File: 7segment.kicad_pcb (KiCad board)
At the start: 2 copper layers, 31.8 x 23.4 mm, 12 parts, among them J1 VCC, J2 IN_UP, J3 GND, J4 IN_DOWN, U1 LTD-2601G, U2 ATmega328P-AU

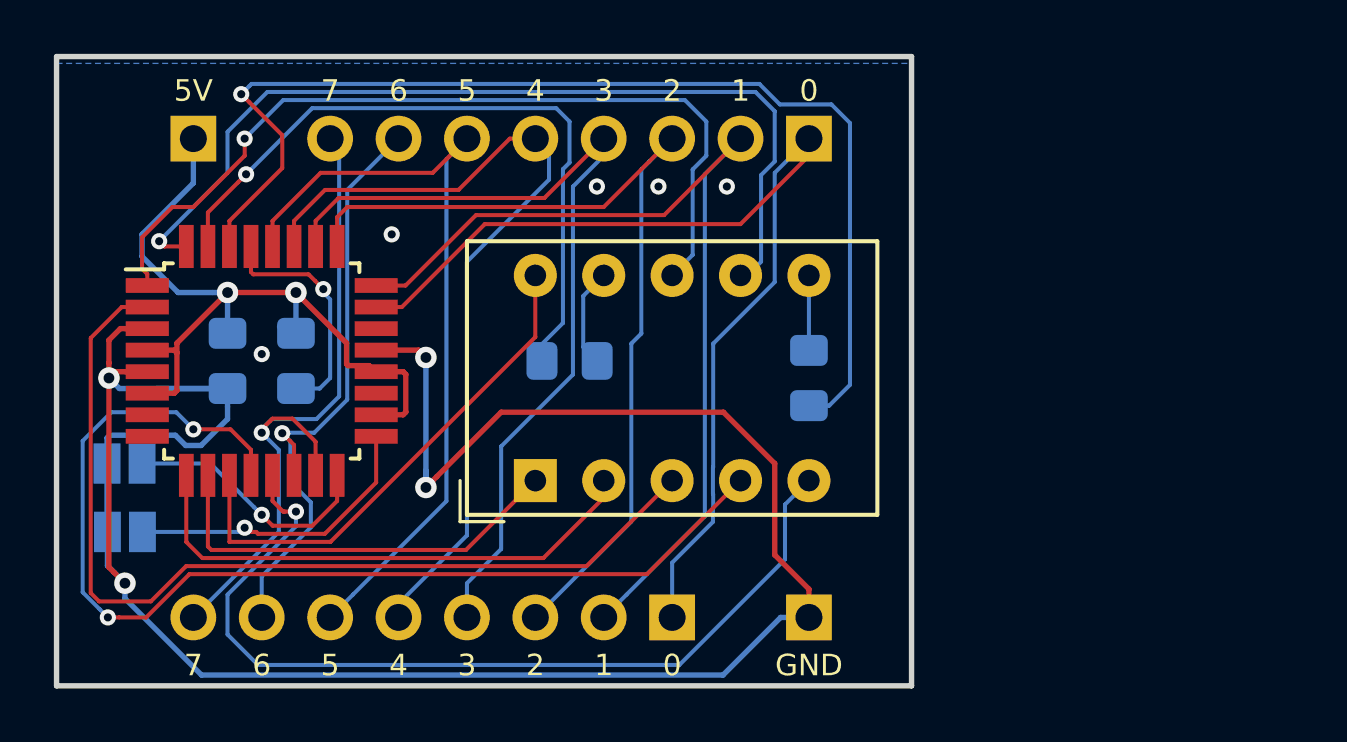
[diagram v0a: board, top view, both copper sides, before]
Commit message: Revision B
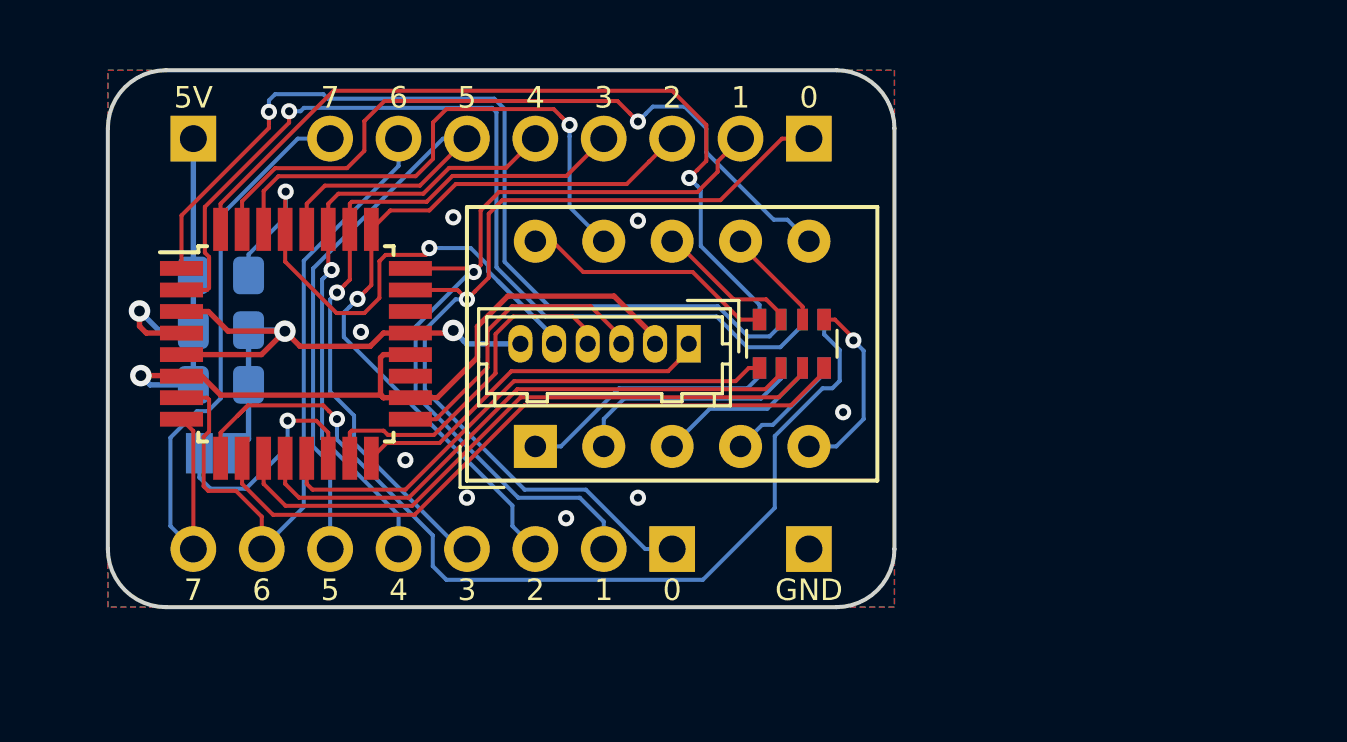
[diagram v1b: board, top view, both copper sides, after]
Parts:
- removed JP1: DIM, Jumper:SolderJumper-2_P1.3mm_Open_Pad1.0x1.5mm
- removed R1, R2: 220, Resistor_SMD:R_0805_2012Metric_Pad1.15x1.40mm_HandSolder
- added C2: 0.1uF, Capacitor_SMD:C_0805_2012Metric_Pad1.15x1.40mm_HandSolder, B.Cu at (64.5, 47.2)
- added J5: AVR-ISP-6, Connector_Hirose:Hirose_DF13-06P-1.25DSA_1x06_P1.25mm_Vertical, F.Cu at (81.9, 45.7)
- added RN1: 220, Resistor_SMD:R_Array_Convex_4x0603, B.Cu at (85.7, 45.7)
- added RN2: 220, Resistor_SMD:R_Array_Convex_4x0603, F.Cu at (85.7, 45.7)
- moved JP2 4.49 mm to (64.4, 49.8), turned to 0 degrees
- moved R3 4.22 mm to (64.5, 43.2), turned to 0 degrees
- moved J3 2.54 mm to (86.4, 53.3), turned to 90 degrees
- moved J4 2.54 mm to (81.3, 53.3)
- moved U2 1.42 mm to (67.3, 45.7)
- moved U1 1.27 mm to (76.2, 49.5)
- moved C1 1.17 mm to (64.5, 45.2), turned to 0 degrees
- turned J1 to 90 degrees
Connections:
- net Net-(R3-Pad2) renamed ~RESET
- U1 pad 1: Net-(U1-Pad1) -> SEG_E
- U1 pad 10: Net-(U1-Pad10) -> SEG_F
- U1 pad 2: Net-(U1-Pad2) -> SEG_D
- U1 pad 3: Net-(U1-Pad3) -> SEG_C
- U1 pad 4: Net-(U1-Pad4) -> SEG_G
- U1 pad 5: Net-(U1-Pad5) -> SEG_DP
- U1 pad 6: Net-(R2-Pad2) -> D1
- U1 pad 7: Net-(U1-Pad7) -> SEG_A
- U1 pad 8: Net-(U1-Pad8) -> SEG_B
- U1 pad 9: Net-(R1-Pad2) -> D0
- U2 pad 1: Net-(U1-Pad8) -> Net-(RN1-Pad2)
- U2 pad 10: Net-(U1-Pad1) -> Net-(RN2-Pad8)
- U2 pad 11: Net-(U1-Pad10) -> Net-(RN2-Pad7)
- U2 pad 12: Net-(U1-Pad4) -> Net-(RN2-Pad6)
- U2 pad 13: Net-(U1-Pad5) -> Net-(RN2-Pad5)
- U2 pad 14: /IN6 -> Net-(JP2-Pad1)
- U2 pad 15: /IN7 -> MOSI
- U2 pad 16: Net-(JP1-Pad1) -> MISO
- U2 pad 17: Net-(JP2-Pad1) -> SCK
- U2 pad 2: Net-(U1-Pad3) -> Net-(RN1-Pad3)
- U2 pad 30: Net-(R2-Pad1) -> D0
- U2 pad 31: Net-(R1-Pad1) -> D1
- U2 pad 32: Net-(U1-Pad7) -> Net-(RN1-Pad1)
- U2 pad 7: Net-(U2-Pad7) -> /IN6
- U2 pad 8: Net-(U2-Pad8) -> /IN7
- U2 pad 9: Net-(U1-Pad2) -> Net-(RN1-Pad4)
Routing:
- net GND: track 89.7 -> 23.9 mm, vias 9 -> 10
- net Net-(R2-Pad1): track 42.0 -> 0.00 mm, vias 1 -> 0
- net Net-(U1-Pad4): track 40.8 -> 0.00 mm, vias 2 -> 0
- net Net-(RN1-Pad4): track 0.00 -> 35.8 mm, vias 0 -> 1
- net Net-(RN1-Pad3): track 0.00 -> 35.7 mm, vias 0 -> 1
- net Net-(U1-Pad3): track 35.6 -> 0.00 mm
- net Net-(U1-Pad7): track 34.2 -> 0.00 mm, vias 1 -> 0
- net Net-(RN1-Pad2): track 0.00 -> 34.1 mm, vias 0 -> 1
- net Net-(U1-Pad5): track 33.7 -> 0.00 mm, vias 1 -> 0
- net Net-(U1-Pad8): track 31.9 -> 0.00 mm, vias 1 -> 0
- net Net-(RN1-Pad1): track 0.00 -> 30.0 mm, vias 0 -> 1
- net D1: track 0.00 -> 27.4 mm, vias 0 -> 1
- net Net-(R1-Pad1): track 25.8 -> 0.00 mm, vias 1 -> 0
- net Net-(RN2-Pad8): track 0.00 -> 25.4 mm
- net Net-(RN2-Pad7): track 0.00 -> 23.5 mm
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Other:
- board size 31.8 x 23.4 mm -> 29.2 x 19.9 mm
- rule pad_to_mask_clearance: 0.12 -> 0.1
- board text added: "MISO"
- board text added: "MOSI"
- board text added: "RevB 2019 dev@hotkeysoft.net"
- board text added: "SCK"
- board text added: "VCC"
- board text added: "~RST"
- board text removed: "8 bit HEX Display RevA 2009 Dominic Thibodeau dev@hotkeysoft.net"
- board text removed: "DIM"

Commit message: Rev C
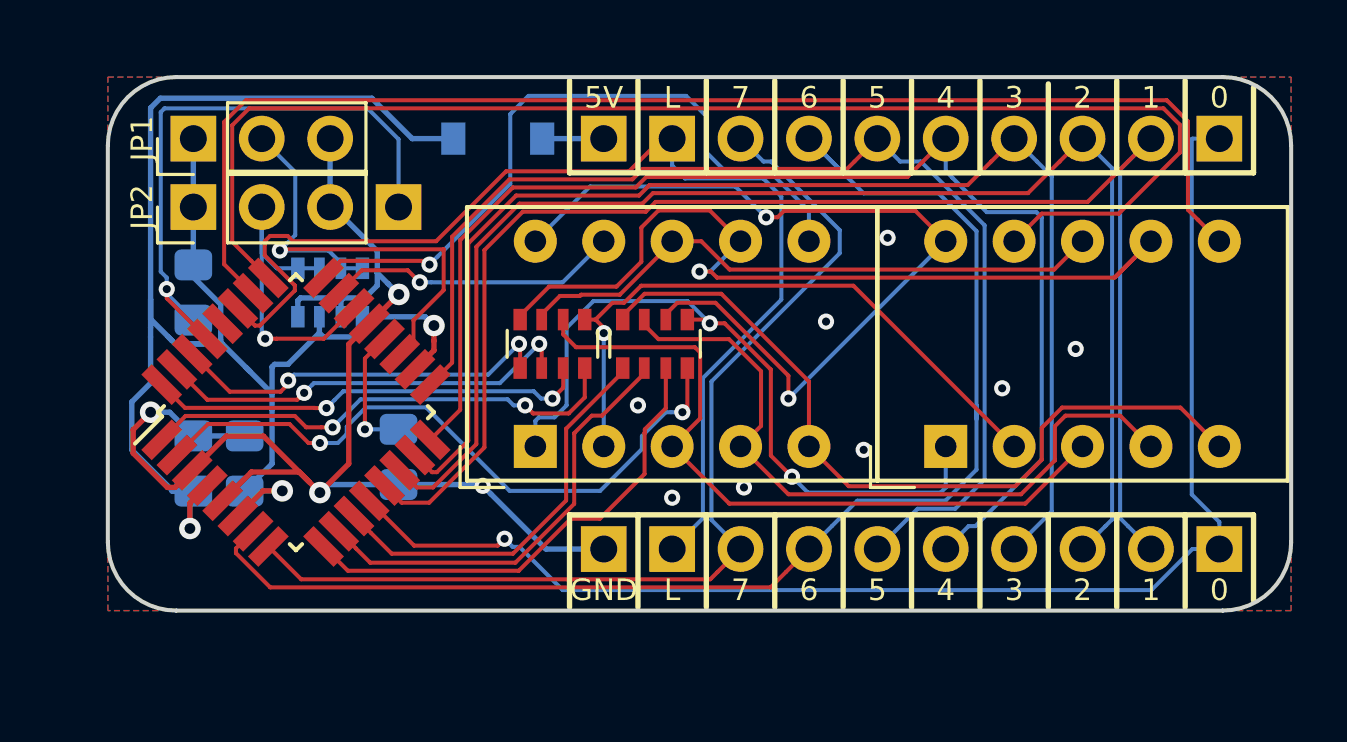
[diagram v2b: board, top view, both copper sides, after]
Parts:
- added C3: 0.1uF, Capacitor_SMD:C_0805_2012Metric_Pad1.15x1.40mm_HandSolder, B.Cu at (71.1, 49.9)
- added D1: MBR0520LT, Diode_SMD:D_SOD-123, B.Cu at (74.8, 38.1)
- added J6: LATCH, Connector_PinHeader_2.54mm:PinHeader_1x01_P2.54mm_Vertical, B.Cu at (81.3, 38.1)
- added J7: LATCH, Connector_PinHeader_2.54mm:PinHeader_1x01_P2.54mm_Vertical, B.Cu at (81.3, 53.3)
- added JP1: BIN/DEC, Connector_PinHeader_2.54mm:PinHeader_1x03_P2.54mm_Vertical, F.Cu at (63.5, 38.1)
- added RN3: 10K, Resistor_SMD:R_Array_Convex_4x0603, B.Cu at (68.6, 43.8)
- added U3: LTD-2601G, DTLib:LTD-2601G, F.Cu at (91.4, 49.5)
- J5: value AVR-ISP-6 -> RESET; footprint Connector_Hirose:Hirose_DF13-06P-1.25DSA_1x06_P1.25mm_Vertical -> Connector_PinHeader_2.54mm:PinHeader_1x01_P2.54mm_Vertical; moved to B.Cu
- JP2: value DEC -> LATCH MODE; footprint Jumper:SolderJumper-2_P1.3mm_Open_Pad1.0x1.5mm -> Connector_PinHeader_2.54mm:PinHeader_1x03_P2.54mm_Vertical; moved to F.Cu
- RN1: value 220 -> 330; moved to F.Cu
- RN2: value 220 -> 330
- moved J4 20.3 mm to (101.6, 53.3)
- moved J1 15.2 mm to (78.7, 38.1), turned to 0 degrees
- moved J2 15.2 mm to (101.6, 38.1)
- moved J5 11.9 mm to (71.1, 40.6), turned to 0 degrees
- moved JP2 9.19 mm to (63.5, 40.6), turned to 90 degrees
- moved RN1 8.89 mm to (76.8, 45.7), turned to 90 degrees
- moved J3 7.62 mm to (78.7, 53.3), turned to 0 degrees
- moved RN2 5.08 mm to (80.6, 45.7)
- moved C1 5.03 mm to (65.4, 50.2), turned to 90 degrees
- moved C2 3.10 mm to (63.5, 50.2), turned to 90 degrees
- moved U2 2.54 mm to (67.3, 48.3), turned to 45 degrees
- moved R3 1.21 mm to (63.5, 43.8), turned to 270 degrees
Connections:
- J1 pad 1: VCC -> /VIN
- J2 pad 4: /IN3 -> MOSI
- J2 pad 5: /IN4 -> MISO
- J2 pad 6: /IN5 -> SCK
- J4 pad 4: /IN3 -> MOSI
- J4 pad 5: /IN4 -> MISO
- J4 pad 6: /IN5 -> SCK
- J5 pad 1: MISO -> ~RESET
- JP2 pad 1: Net-(JP2-Pad1) -> VCC
- JP2 pad 2: GND -> SEL_LATCHMODE
- RN1 pad 5: SEG_G -> SEG_D
- RN1 pad 7: SEG_D -> SEG_B
- RN1 pad 8: SEG_E -> SEG_A
- RN2 pad 1: SEG_DP -> SEG_E
- RN2 pad 2: SEG_A -> SEG_F
- RN2 pad 3: SEG_B -> SEG_G
- RN2 pad 4: SEG_F -> SEG_DP
- U2 pad 1: Net-(RN1-Pad2) -> Net-(RN1-Pad4)
- U2 pad 10: Net-(RN2-Pad8) -> Net-(RN2-Pad6)
- U2 pad 11: Net-(RN2-Pad7) -> Net-(RN2-Pad5)
- U2 pad 12: Net-(RN2-Pad6) -> /IN0
- U2 pad 13: Net-(RN2-Pad5) -> /IN1
- U2 pad 14: Net-(JP2-Pad1) -> /IN2
- U2 pad 19: Net-(U2-Pad19) -> SEL_NUMBERBASE
- U2 pad 2: Net-(RN1-Pad3) -> Net-(RN2-Pad8)
- U2 pad 20: VCC -> Net-(C3-Pad2)
- U2 pad 22: Net-(U2-Pad22) -> SEL_LATCHMODE
- U2 pad 23: /IN0 -> D0
- U2 pad 24: /IN1 -> D1
- U2 pad 25: /IN2 -> D2
- U2 pad 26: /IN3 -> D3
- U2 pad 27: /IN4 -> Net-(J6-Pad1)
- U2 pad 28: /IN5 -> Net-(U2-Pad28)
- U2 pad 30: D0 -> Net-(RN1-Pad1)
- U2 pad 31: D1 -> Net-(RN1-Pad2)
- U2 pad 32: Net-(RN1-Pad1) -> Net-(RN1-Pad3)
- U2 pad 9: Net-(RN1-Pad4) -> Net-(RN2-Pad7)
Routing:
- net D2: track 0.00 -> 50.5 mm
- net D3: track 0.00 -> 48.2 mm
- net Net-(J6-Pad1): track 0.00 -> 42.4 mm
- net MOSI: track 13.5 -> 48.3 mm
- net MISO: track 13.7 -> 46.9 mm
- net SCK: track 11.1 -> 42.9 mm
- net SEG_A: track 3.86 -> 32.5 mm, vias 0 -> 1
- net GND: track 23.9 -> 50.6 mm, vias 10 -> 12
- net /IN5: track 26.3 -> 0.00 mm
- net /IN3: track 25.8 -> 0.00 mm, vias 1 -> 0
- net VCC: track 41.1 -> 66.2 mm, vias 2 -> 3
- net /IN6: track 25.5 -> 50.1 mm
- net /IN2: track 27.8 -> 51.4 mm, vias 1 -> 0
- net /IN1: track 31.3 -> 54.8 mm, vias 1 -> 0
- net /IN4: track 22.9 -> 0.00 mm, vias 1 -> 0
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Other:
- board size 29.2 x 19.9 mm -> 43.9 x 19.8 mm
- board text added: "1-2 2-3 OFF"
- board text added: "8 bit DEC/HEX Display RevC 2019 Dominic Thibodeau dev@hotkeysoft.net"
- board text added: "DECIMAL (SIGNED) DECIMAL (UNSIGNED) HEXADECIMAL"
- board text added: "JP1: DEC/HEX"
- board text added: "JP2: LATCH"
- board text added: "L"
- board text added: "LATCH L->H LATCH H->L NOT LATCHED"
- board text added: "POS"
- board text removed: "DECIMAL"
- board text removed: "RevB 2019 dev@hotkeysoft.net"
